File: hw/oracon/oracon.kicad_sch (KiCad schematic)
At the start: 104 parts, among them J2 SIM_Card, J3 USB_A, J4 Conn_Coaxial, J5 USB_C_Receptacle_USB2.0_16P, Q1 SS8050, Q2 SS8050, Q3 SS8050, Q5 SS8050, SW1 SW_Push, U1 TP5100, U2 AMS1117-3.3, U3 ESP32-S3-MINI-1U, U4 CH343P, U5 TPS61022, U6 MAX3232, U7 SIM7022

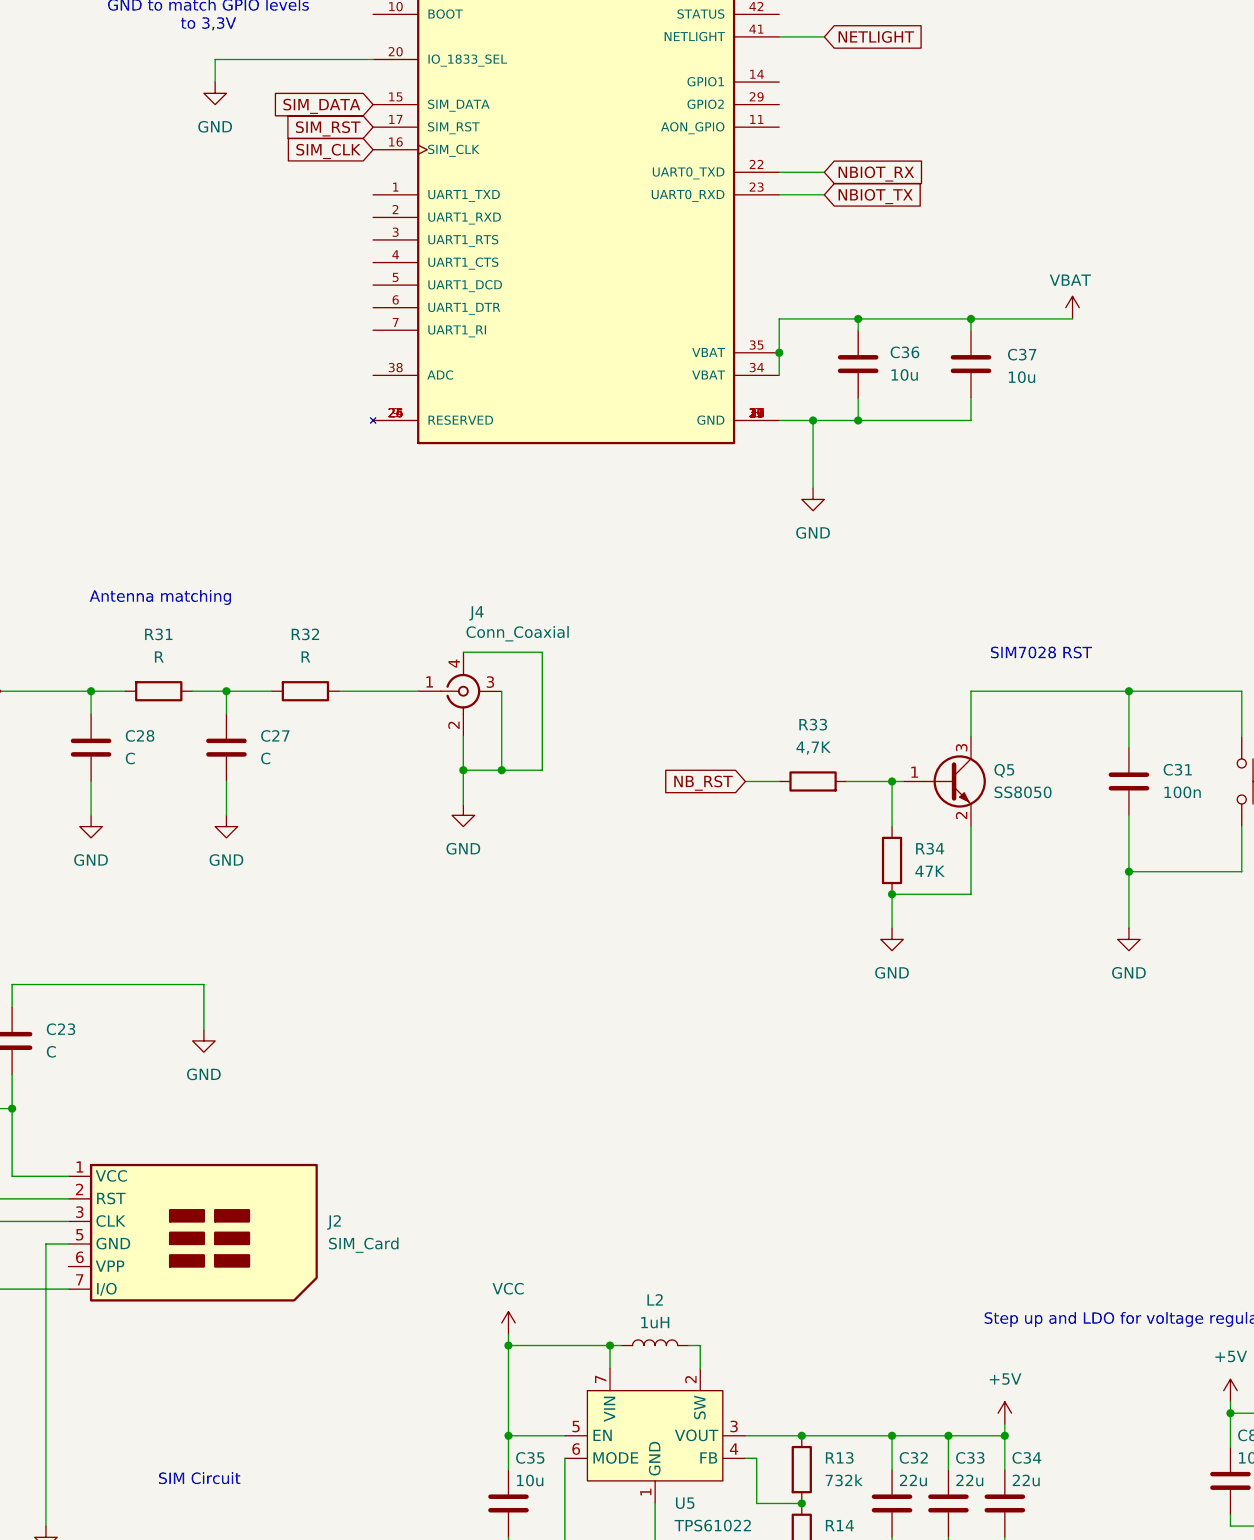
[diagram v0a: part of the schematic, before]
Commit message: PCB work, paths and zones
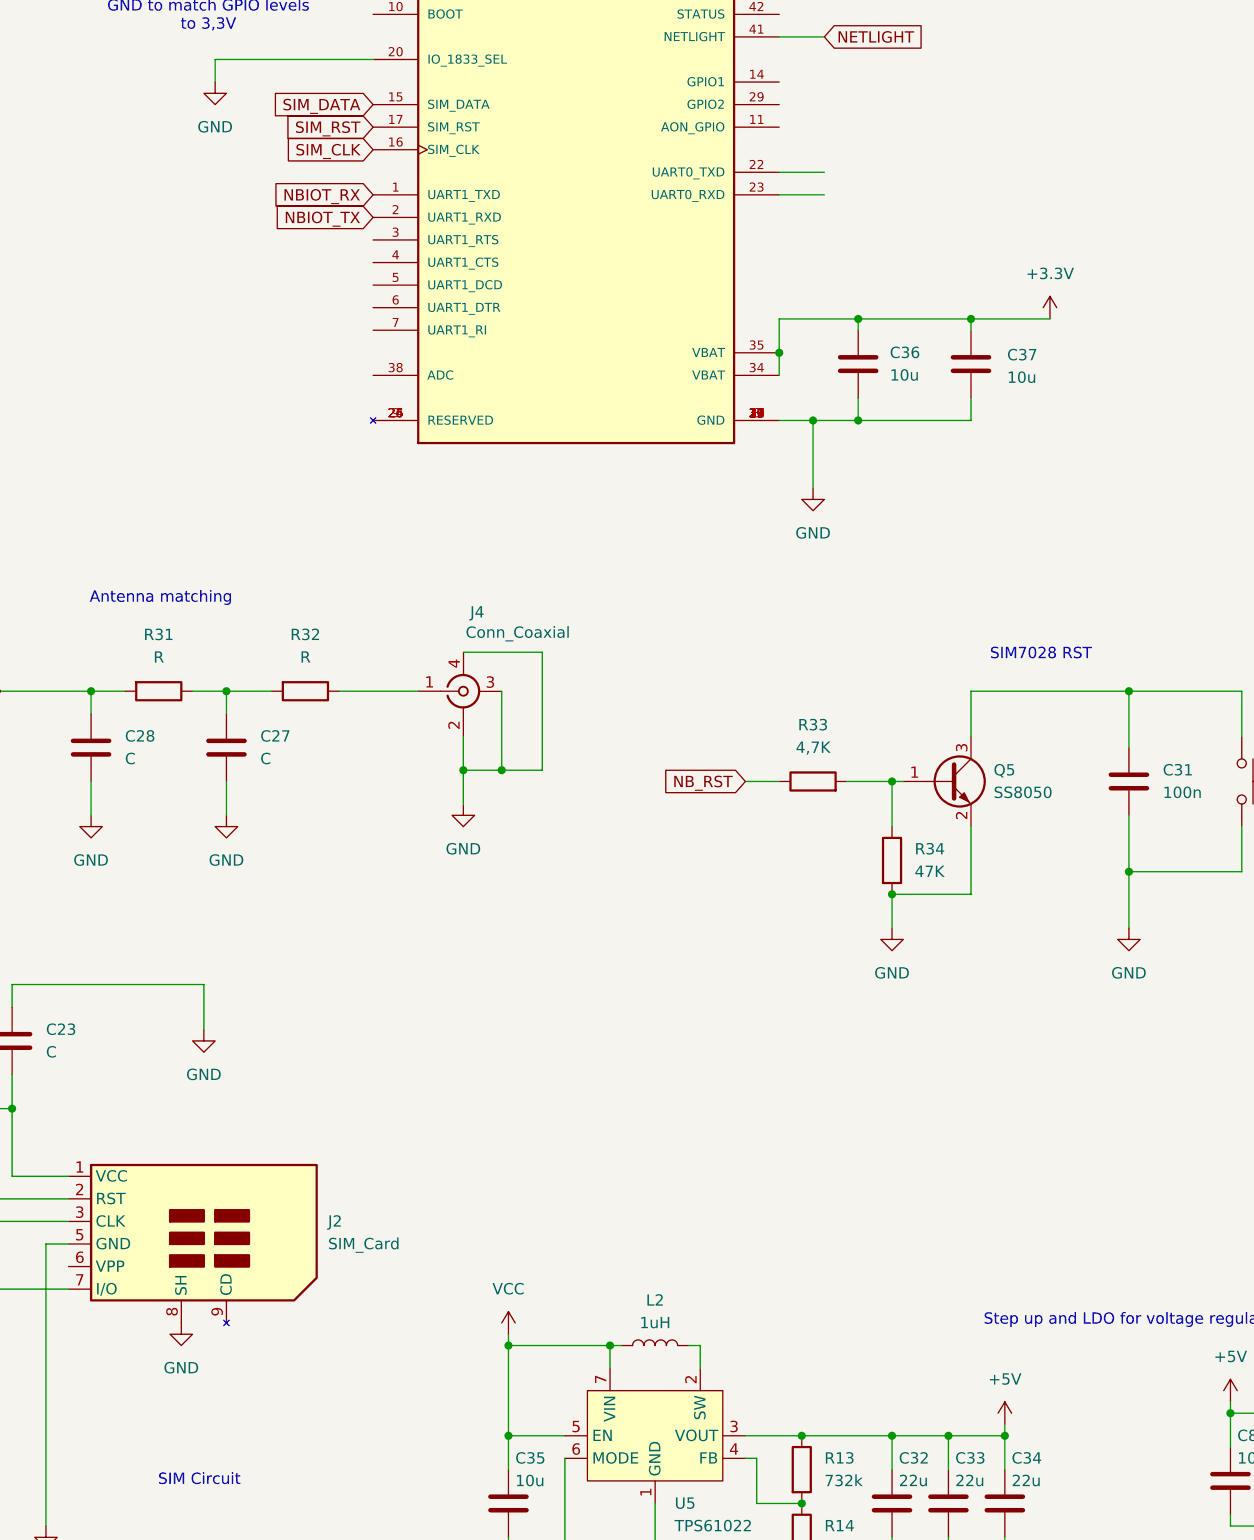
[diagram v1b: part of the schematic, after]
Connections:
- net VBAT is gone; now on net +3.3V: C36.1, C37.1, U7.34 (VBAT), U7.35 (VBAT)
- net GND: now also J2.8 (SH)
- net NBIOT_RX: now also U7.1 (UART1_TXD); no longer U7.22 (UART0_TXD)
- net NBIOT_TX: now also U7.2 (UART1_RXD); no longer U7.23 (UART0_RXD)
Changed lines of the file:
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@@
 	(wire
 		(pts
-			(xy 219.71 135.89) (xy 208.28 135.89)
-		)
-		(stroke
-			(width 0)
-			(type default)
-		)
-	)
-	(wire
-		(pts
 			(xy 175.26 31.75) (xy 144.78 31.75)
 		)
@@
 	(wire
 		(pts
+			(xy 217.17 135.89) (xy 208.28 135.89)
+		)
+		(stroke
+			(width 0)
+			(type default)
+		)
+	)
+	(wire
+		(pts
 			(xy 276.86 73.66) (xy 311.15 73.66)
 		)
@@
 		)
 	)
+	(global_label "NBIOT_RX"
+		(shape input)
+		(at 140.97 121.92 180)
+		(fields_autoplaced yes)
+		(effects
+			(font
+				(size 1.27 1.27)
+			)
+			(justify right)
+		)
+		(property "Intersheetrefs" "${INTERSHEET_REFS}"
+			(at 129.0343 121.92 0)
+			(effects
+				(font
+					(size 1.27 1.27)
+				)
+				(justify right)
+				(hide yes)
+			)
+		)
+	)
 	(global_label "LED3_B"
 		(shape input)
@@
 		)
 	)
-	(global_label "NBIOT_TX"
+	(global_label "LED1_B"
 		(shape input)
-		(at 191.77 121.92 0)
+		(at 78.74 137.16 0)
 		(fields_autoplaced yes)
 		(effects
@@
 		)
 		(property "Intersheetrefs" "${INTERSHEET_REFS}"
-			(at 203.4033 121.92 0)
+			(at 88.6194 137.16 0)
 			(effects
 				(font
@@
 		)
 	)
-	(global_label "LED1_B"
+	(global_label "USB_SI_N"
 		(shape input)
-		(at 78.74 137.16 0)
+		(at 48.26 109.22 180)
 		(fields_autoplaced yes)
 		(effects
@@
 				(size 1.27 1.27)
 			)
-			(justify left)
+			(justify right)
 		)
 		(property "Intersheetrefs" "${INTERSHEET_REFS}"
-			(at 88.6194 137.16 0)
+			(at 36.3848 109.22 0)
 			(effects
 				(font
 					(size 1.27 1.27)
 				)
-				(justify left)
+				(justify right)
 				(hide yes)
 			)
 		)
 	)
-	(global_label "USB_SI_N"
+	(global_label "NBIOT_TX"
 		(shape input)
-		(at 48.26 109.22 180)
+		(at 140.97 124.46 180)
 		(fields_autoplaced yes)
 		(effects
@@
 		)
 		(property "Intersheetrefs" "${INTERSHEET_REFS}"
-			(at 36.3848 109.22 0)
+			(at 129.3367 124.46 0)
 			(effects
 				(font
@@
 		)
 	)
-	(global_label "NBIOT_RX"
-		(shape input)
-		(at 191.77 119.38 0)
-		(fields_autoplaced yes)
-		(effects
-			(font
-				(size 1.27 1.27)
-			)
-			(justify left)
-		)
-		(property "Intersheetrefs" "${INTERSHEET_REFS}"
-			(at 203.7057 119.38 0)
-			(effects
-				(font
-					(size 1.27 1.27)
-				)
-				(justify left)
-				(hide yes)
-			)
-		)
-	)
 	(global_label "LED2_B"
 		(shape input)
@@
 	(symbol
 		(lib_id "power:GND")
+		(at 119.38 248.92 0)
+		(unit 1)
+		(exclude_from_sim no)
+		(in_bom yes)
+		(on_board yes)
+		(dnp no)
+		(fields_autoplaced yes)
+		(property "Reference" "#PWR030"
+			(at 119.38 255.27 0)
+			(effects
+				(font
+					(size 1.27 1.27)
+				)
+				(hide yes)
+			)
+		)
+		(property "Value" "GND"
+			(at 119.38 254 0)
+			(effects
+				(font
+					(size 1.27 1.27)
+				)
+			)
+		)
+		(property "Footprint" ""
+			(at 119.38 248.92 0)
+			(effects
+				(font
+					(size 1.27 1.27)
+				)
+				(hide yes)
+			)
+		)
+		(property "Datasheet" ""
+			(at 119.38 248.92 0)
+			(effects
+				(font
+					(size 1.27 1.27)
+				)
+				(hide yes)
+			)
+		)
+		(property "Description" "Power symbol creates a global label with name \"GND\" , ground"
+			(at 119.38 248.92 0)
+			(effects
+				(font
+					(size 1.27 1.27)
+				)
+				(hide yes)
+			)
+		)
+		(pin "1"
+		)
+		(instances
+			(project "oracon"
+				(path "/7501ec1f-5c34-40ce-b7e3-cacc6e1961d1"
+					(reference "#PWR030")
+					(unit 1)
+				)
+			)
+		)
+	)
+	(symbol
+		(lib_id "power:GND")
 		(at 190.5 154.94 0)
 		(unit 1)
@@
 	)
 	(symbol
+		(lib_id "power:+3.3V")
+		(at 217.17 135.89 0)
+		(unit 1)
+		(exclude_from_sim no)
+		(in_bom yes)
+		(on_board yes)
+		(dnp no)
+		(fields_autoplaced yes)
+		(property "Reference" "#PWR050"
+			(at 217.17 139.7 0)
+			(effects
+				(font
+					(size 1.27 1.27)
+				)
+				(hide yes)
+			)
+		)
+		(property "Value" "+3.3V"
+			(at 217.17 130.81 0)
+			(effects
+				(font
+					(size 1.27 1.27)
+				)
+			)
+		)
+		(property "Footprint" ""
+			(at 217.17 135.89 0)
+			(effects
+				(font
+					(size 1.27 1.27)
+				)
+				(hide yes)
+			)
+		)
+		(property "Datasheet" ""
+			(at 217.17 135.89 0)
+			(effects
+				(font
+					(size 1.27 1.27)
+				)
+				(hide yes)
+			)
+		)
+		(property "Description" "Power symbol creates a global label with name \"+3.3V\""
+			(at 217.17 135.89 0)
+			(effects
+				(font
+					(size 1.27 1.27)
+				)
+				(hide yes)
+			)
+		)
+		(pin "1"
+		)
+		(instances
+			(project "oracon"
+				(path "/7501ec1f-5c34-40ce-b7e3-cacc6e1961d1"
+					(reference "#PWR050")
+					(unit 1)
+				)
+			)
+		)
+	)
+	(symbol
 		(lib_id "Device:C")
 		(at 124.46 184.15 0)
@@
 	)
 	(symbol
-		(lib_id "power:+3.3V")
-		(at 219.71 135.89 0)
-		(unit 1)
-		(exclude_from_sim no)
-		(in_bom yes)
-		(on_board yes)
-		(dnp no)
-		(property "Reference" "#PWR051"
-			(at 219.71 139.7 0)
-			(effects
-				(font
-					(size 1.27 1.27)
-				)
-				(hide yes)
-			)
-		)
-		(property "Value" "VBAT"
-			(at 219.456 131.572 0)
-			(effects
-				(font
-					(size 1.27 1.27)
-				)
-			)
-		)
-		(property "Footprint" ""
-			(at 219.71 135.89 0)
-			(effects
-				(font
-					(size 1.27 1.27)
-				)
-				(hide yes)
-			)
-		)
-		(property "Datasheet" ""
-			(at 219.71 135.89 0)
-			(effects
-				(font
-					(size 1.27 1.27)
-				)
-				(hide yes)
-			)
-		)
-		(property "Description" "Power symbol creates a global label with name \"+3.3V\""
-			(at 219.71 135.89 0)
-			(effects
-				(font
-					(size 1.27 1.27)
-				)
-				(hide yes)
-			)
-		)
-		(pin "1"
-		)
-		(instances
-			(project "nbiot_esp32s3_hat"
-				(path "/7501ec1f-5c34-40ce-b7e3-cacc6e1961d1"
-					(reference "#PWR051")
-					(unit 1)
-				)
-			)
-		)
-	)
-	(symbol
 		(lib_id "Transistor_BJT:SS8050")
 		(at 327.66 25.4 0)
@@
 		(pin "2"
 		)
+		(pin "8"
+		)
+		(pin "9"
+		)
 		(instances
